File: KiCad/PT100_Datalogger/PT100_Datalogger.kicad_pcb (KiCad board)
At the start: 4 copper layers, 90 x 122 mm, 190 parts, among them J1 PWR, J10 Conn_01x03, J11 Conn_01x03, J12 Conn_01x03, J13 HLK-LD2410C, J14 691406710003B, J2 USB_C_Receptacle, J3 Screw_Terminal_01x02, J4 CT, J5 SJ1-3523N, J6 JTAG, J7 CT_SW, J8 Conn_01x03, J9 Conn_01x03, K1 J115F11CH5VDCS61.5U, Q10 BSS806NEH6327XTSA1, Q11 SSM3J36FS,LF, Q12 SSM3J36FS,LF, Q13 SSM3J36FS,LF, Q14 BSS806NEH6327XTSA1, Q15 SSM3J36FS,LF, Q16 MMBT3904, Q17 MMBT3904, Q3 BSS806NEH6327XTSA1, Q4 BSS806NEH6327XTSA1, Q5 BSS806NEH6327XTSA1, Q6 BSS806NEH6327XTSA1, Q7 BSS806NEH6327XTSA1, Q8 BSS806NEH6327XTSA1, Q9 BSS806NEH6327XTSA1, SW3 SW_Push_Shielded, SW4 SW_Push_Shielded, SW5 SW_Push_Shielded, SW6 SW_Push_Shielded, SW7 SW_Push_Shielded, U1 ESP32-S3-WROOM-1-N8R2, U10 SHT4x, U11 PCF85263AT, U12 FM24CL16B-GTR, U13 MCP9601, U2 CP2102N-Axx-xQFN28, U3 NCS2250SQ2T2G, U4 LDL212PV33R, U5 TMP1075DSG, U6 INND-TS56RAB, U7 INND-TS56RAB, U8 INND-TS56RAB, U9 INND-TS56RAB, Y1 32.768K12.5PI/3215E

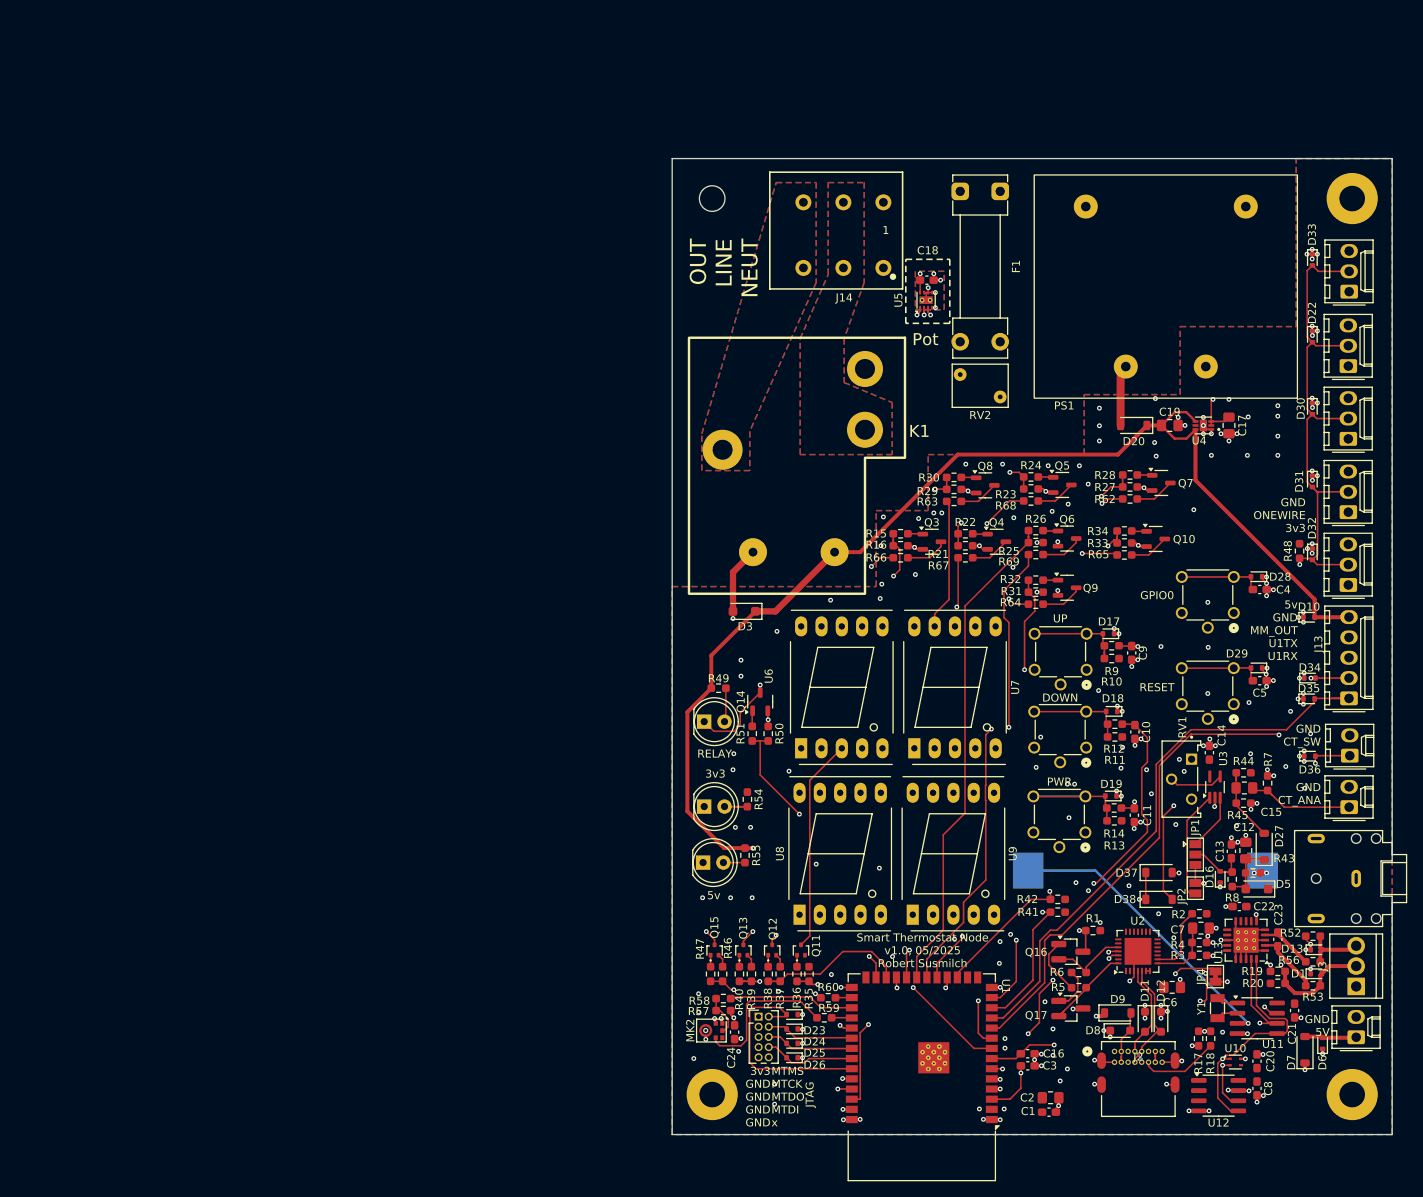
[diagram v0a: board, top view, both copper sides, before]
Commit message: Finished KiCad PCB REV A
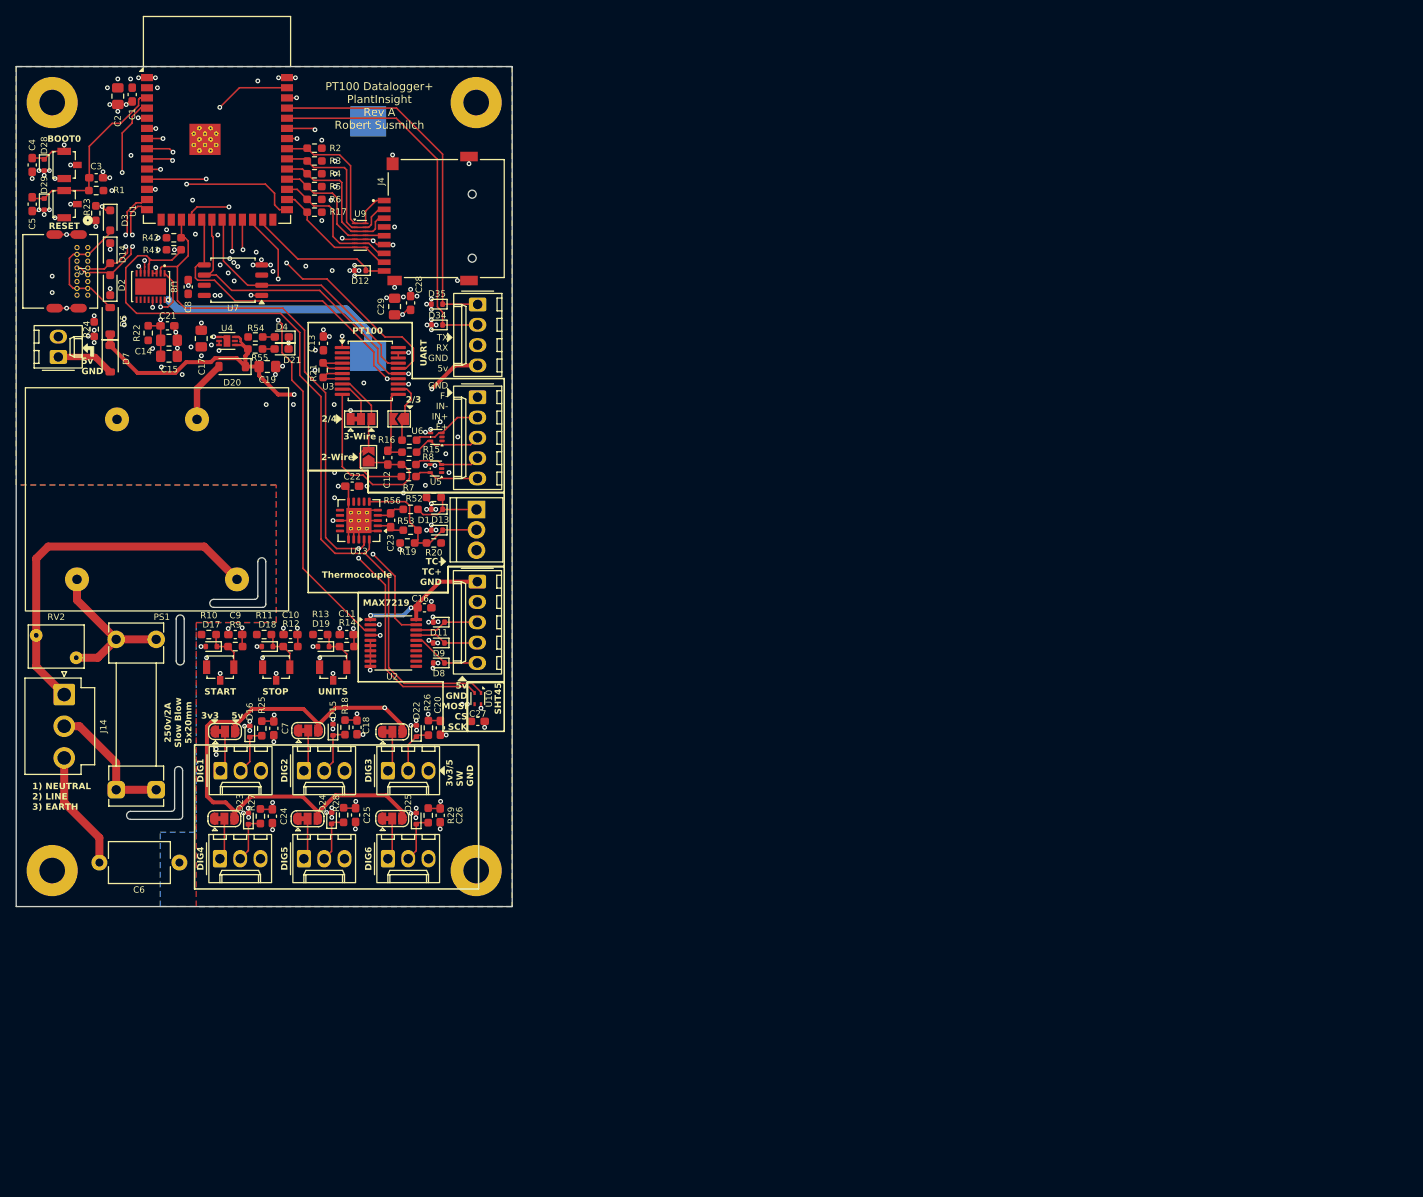
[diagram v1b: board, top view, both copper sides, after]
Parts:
- removed D10, D6: ESD5Z12T1G, Diode_SMD:D_SOD-523
- removed D26, D30, D31, D32, D33, D36: ESD5Z3V3, Diode_SMD:D_SOD-523
- removed D27, D37, D38: B5819W, Diode_SMD:D_SOD-123
- removed K1: J115F11CH5VDCS61.5U, Personal:J115FX
- removed MK2: ICS-43434, Sensor_Audio:InvenSense_ICS-43434-6_3.5x2.65mm
- removed Q10, Q14, Q3, Q4, Q5, Q6, Q7, Q8, Q9: BSS806NEH6327XTSA1, Package_TO_SOT_SMD:SOT-23-3
- removed Q11, Q12, Q13, Q15: SSM3J36FS,LF, Package_TO_SOT_SMD:SOT-416
- removed Q16, Q17: MMBT3904, Package_TO_SOT_SMD:SOT-23_Handsoldering
- removed R30, R32, R34, R36, R38, R40, R47, R51: 1K, Resistor_SMD:R_0603_1608Metric_Pad0.98x0.95mm_HandSolder
- removed R31, R33, R35, R37, R39, R46, R50, R57: 100K, Resistor_SMD:R_0603_1608Metric_Pad0.98x0.95mm_HandSolder
- removed R43: 1M, Resistor_SMD:R_0603_1608Metric_Pad0.98x0.95mm_HandSolder
- removed R44, R45: 10k, Resistor_SMD:R_0603_1608Metric_Pad0.98x0.95mm_HandSolder
- removed R48: 4K7, Resistor_SMD:R_0603_1608Metric_Pad0.98x0.95mm_HandSolder
- removed R49: 220R, Resistor_SMD:R_0603_1608Metric_Pad0.98x0.95mm_HandSolder
- removed R58, R59, R60: 51R, Resistor_SMD:R_0603_1608Metric_Pad0.98x0.95mm_HandSolder
- removed R62, R63, R64, R65, R66, R67, R68, R69: 22R, Resistor_SMD:R_0603_1608Metric_Pad0.98x0.95mm_HandSolder
- removed RV1: PV36Y102C01B00, Personal:TRIM_PV36Y102C01B00
- removed U11: PCF85263AT, Package_SO:SOIC-8_3.9x4.9mm_P1.27mm
- removed U12: FM24CL16B-GTR, Package_SO:SOIC-8_3.9x4.9mm_P1.27mm
- removed Y1: 32.768K12.5PI/3215E, Crystal:Crystal_SMD_3215-2Pin_3.2x1.5mm
- added C25: 100nF, Capacitor_SMD:C_0603_1608Metric_Pad1.08x0.95mm_HandSolder, F.Cu at (94.4, 141.1)
- added C26: 100nF, Capacitor_SMD:C_0603_1608Metric_Pad1.08x0.95mm_HandSolder, F.Cu at (105.0, 141.1)
- added C27: 100nF, Capacitor_SMD:C_0603_1608Metric_Pad1.08x0.95mm_HandSolder, F.Cu at (109.7, 129.3)
- added C28: 100nF, Capacitor_SMD:C_0603_1608Metric_Pad1.08x0.95mm_HandSolder, F.Cu at (101.3, 77.0)
- added C29: 10uF, Capacitor_SMD:C_0805_2012Metric_Pad1.18x1.45mm_HandSolder, F.Cu at (99.3, 77.5)
- added D14: TSD05CDYFR, Diode_SMD:D_SOD-323_HandSoldering, F.Cu at (63.8, 70.8)
- added D15: ESD5Z3V3, Diode_SMD:D_SOD-523, F.Cu at (91.6, 130.4)
- added JP3: SolderJumper_3_Bridged12, Jumper:SolderJumper-3_P1.3mm_Bridged12_RoundedPad1.0x1.5mm, F.Cu at (99.0, 130.7)
- added JP5: SolderJumper_3_Bridged12, Jumper:SolderJumper-3_P1.3mm_Bridged12_RoundedPad1.0x1.5mm, F.Cu at (88.4, 141.5)
- added JP6: SolderJumper_3_Bridged12, Jumper:SolderJumper-3_P1.3mm_Bridged12_RoundedPad1.0x1.5mm, F.Cu at (99.0, 141.5)
- added JP7: SolderJumper_3_Bridged12, Jumper:SolderJumper-3_P1.3mm_Bridged12_Pad1.0x1.5mm, F.Cu at (95.1, 91.6)
- added JP8: SolderJumper_2_Open, Jumper:SolderJumper-2_P1.3mm_Open_TrianglePad1.0x1.5mm, F.Cu at (99.9, 91.5)
- added JP9: SolderJumper_2_Open, Jumper:SolderJumper-2_P1.3mm_Open_TrianglePad1.0x1.5mm, F.Cu at (96.0, 96.3)
- C12, C7: value 10uF -> 100nF; footprint Capacitor_SMD:C_0805_2012Metric_Pad1.18x1.45mm_HandSolder -> Capacitor_SMD:C_0603_1608Metric_Pad1.08x0.95mm_HandSolder
- C14: value 100nF -> 22uF; footprint Capacitor_SMD:C_0603_1608Metric_Pad1.08x0.95mm_HandSolder -> Capacitor_SMD:C_0805_2012Metric_Pad1.18x1.45mm_HandSolder
- C15: value 10uF -> 22uF
- C6: value 10uF -> DE1B3RA471KN4AP01F; footprint Capacitor_SMD:C_0805_2012Metric_Pad1.18x1.45mm_HandSolder -> Capacitor_THT:C_Disc_D7.5mm_W5.0mm_P10.00mm
- D11, D8: value TSD05CDYFR -> ESD5Z12T1G; footprint Diode_SMD:D_SOD-323_HandSoldering -> Diode_SMD:D_SOD-523
- D12: value TSD05CDYFR -> ESD5Z3V3; footprint Diode_SMD:D_SOD-323_HandSoldering -> Diode_SMD:D_SOD-523
- D2: value LED -> TSD05CDYFR; footprint LED_THT:LED_D5.0mm -> Diode_SMD:D_SOD-323_HandSoldering
- D21, D4: footprint LED_THT:LED_D5.0mm -> LED_SMD:LED_0603_1608Metric_Pad1.05x0.95mm_HandSolder
- D3: value SM4007PL -> TSD05CDYFR; footprint Diode_SMD:D_SOD-123F -> Diode_SMD:D_SOD-323_HandSoldering
- D5: value SM4007PL -> B5819W; footprint Diode_SMD:D_SOD-123F -> Diode_SMD:D_SOD-123
- D9: value B5819W -> ESD5Z12T1G; footprint Diode_SMD:D_SOD-123 -> Diode_SMD:D_SOD-523
- H1: footprint MountingHole:MountingHole_3.2mm_M3 -> MountingHole:MountingHole_3.2mm_M3_Pad
- J10: value Conn_01x03 -> DIG3
- J11: value Conn_01x03 -> DIG4
- J12: value Conn_01x03 -> DIG5
- J13: value HLK-LD2410C -> DIG6; footprint Connector_Molex:Molex_KK-254_AE-6410-05A_1x05_P2.54mm_Vertical -> Connector_Molex:Molex_KK-254_AE-6410-03A_1x03_P2.54mm_Vertical
- J14: value 691406710003B -> PWR; footprint Personal:691406710003B -> Connector_JST:JST_VH_B3P-VH_1x03_P3.96mm_Vertical
- J2: value USB_C_Receptacle -> Conn_01x04; footprint Personal:CONN_CU3216SASBLR004-NH_CVI -> Connector_Molex:Molex_KK-254_AE-6410-04A_1x04_P2.54mm_Vertical
- J3: value Screw_Terminal_01x02 -> TC
- J4: value CT -> MSD-4-A; footprint Connector_Molex:Molex_KK-254_AE-6410-02A_1x02_P2.54mm_Vertical -> Personal:CUI_MSD-4-A
- J5: value SJ1-3523N -> CU3216SASBLR004-NH; footprint Connector_Audio:Jack_3.5mm_CUI_SJ1-3523N_Horizontal -> Personal:CONN_CU3216SASBLR004-NH_CVI
- J6: value JTAG -> RTD; footprint Connector_PinHeader_1.27mm:PinHeader_2x05_P1.27mm_Vertical -> Connector_Molex:Molex_KK-254_AE-6410-05A_1x05_P2.54mm_Vertical
- J7: value CT_SW -> MAX7219; footprint Connector_Molex:Molex_KK-254_AE-6410-02A_1x02_P2.54mm_Vertical -> Connector_Molex:Molex_KK-254_AE-6410-05A_1x05_P2.54mm_Vertical
- J8: value Conn_01x03 -> DIG1
- J9: value Conn_01x03 -> DIG2
- JP1: value SolderJumper_3_Open -> SolderJumper_3_Bridged12; footprint Jumper:SolderJumper-3_P1.3mm_Open_Pad1.0x1.5mm -> Jumper:SolderJumper-3_P1.3mm_Bridged12_RoundedPad1.0x1.5mm
- JP2: value SolderJumper_2_Open -> SolderJumper_3_Bridged12; footprint Jumper:SolderJumper-2_P1.3mm_Open_Pad1.0x1.5mm -> Jumper:SolderJumper-3_P1.3mm_Bridged12_RoundedPad1.0x1.5mm
- JP4: value SolderJumper_2_Bridged -> SolderJumper_3_Bridged12; footprint Jumper:SolderJumper-2_P1.3mm_Bridged_Pad1.0x1.5mm -> Jumper:SolderJumper-3_P1.3mm_Bridged12_RoundedPad1.0x1.5mm
- R15, R26, R28: value 1K -> 100R
- R16, R25, R27, R29: value 100K -> 100R
- R17: value 5k1 -> 10K
- R18: value 5k1 -> 100R
- R2: value 1K -> 10K
- R21: value 100K -> RN73H1JTTD3920A05
- R22: value 1K -> 330R
- R23: value 100K -> 5k1
- R24: value 1K -> 5k1
- R3: value 22K1 -> 10K
- R4: value 47K5 -> 10K
- R7: value 50R -> 100R
- R8: value 100 -> 100R
- SW3, SW4, SW5, SW6, SW7: footprint Personal:SW_1825955-6_TEC -> Button_Switch_SMD:SW_SPST_B3U-1100P
- U10: value SHT4x -> SHT45
- U2: value CP2102N-Axx-xQFN28 -> SN74LVC245APW; footprint Package_DFN_QFN:QFN-28-1EP_5x5mm_P0.5mm_EP3.35x3.35mm -> Package_SO:TSSOP-20_4.4x6.5mm_P0.65mm
- U3: value NCS2250SQ2T2G -> MAX31865xAP; footprint Package_TO_SOT_SMD:SOT-353_SC-70-5_Handsoldering -> Package_SO:SSOP-20_5.3x7.2mm_P0.65mm
- U5: value TMP1075DSG -> TPD2E001; footprint Package_SON:WSON-8-1EP_2x2mm_P0.5mm_EP0.9x1.6mm_ThermalVias -> Package_TO_SOT_SMD:SOT-553
- U6: value INND-TS56RAB -> TPD2E001; footprint Display_7Segment:7SegmentLED_LTS6760_LTS6780 -> Package_TO_SOT_SMD:SOT-553
- U7: value INND-TS56RAB -> CY15B104QN-50SXI; footprint Display_7Segment:7SegmentLED_LTS6760_LTS6780 -> Package_SO:SOIC-8_5.3x5.3mm_P1.27mm
- U8: value INND-TS56RAB -> PCF2131; footprint Display_7Segment:7SegmentLED_LTS6760_LTS6780 -> Personal:16-HLSON
- U9: value INND-TS56RAB -> TPD6E05U06RVZ; footprint Display_7Segment:7SegmentLED_LTS6760_LTS6780 -> Package_SON:Texas_R-PUSON-N14
- moved J1 183.2 mm to (57.3, 83.8)
- moved J5 177.1 mm to (61.0, 70.1), turned to -90 degrees
- moved D7 172.5 mm to (63.8, 84.0), turned to -90 degrees
- moved C1 171.2 mm to (66.5, 51.0), turned to -90 degrees
- moved C2 171.1 mm to (64.7, 51.2), turned to -90 degrees
- moved C8 167.0 mm to (73.5, 75.0), turned to 90 degrees
- moved H3 164.9 mm to (56.5, 148.0)
- moved C21 164.9 mm to (70.9, 79.9), turned to 0 degrees
- moved C5 164.6 mm to (54.0, 64.7), turned to -90 degrees
- moved C4 162.4 mm to (54.0, 59.8), turned to -90 degrees
- moved D29 162.3 mm to (55.5, 64.7), turned to -90 degrees
- moved C3 160.9 mm to (62.0, 61.4)
- moved D28 160.1 mm to (55.5, 59.8), turned to -90 degrees
- moved D5 160.0 mm to (63.8, 79.3), turned to 90 degrees
- moved R1 155.2 mm to (62.0, 63.0)
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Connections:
- C10 pad 1: TEMP_DOWN -> STOP
- C11 pad 1: SOFT_ON_OFF -> UNITS
- C12 pad 1: Net-(D27-K) -> Net-(JP9-A)
- C12 pad 2: GND -> Net-(JP8-B)
- C13 pad 1: Net-(D16-A2) -> +3V3
- C14 pad 1: +3V3 -> Net-(U8-IFS)
- C15 pad 1: Net-(J4-Pin_1) -> Net-(U8-IFS)
- C15 pad 2: Net-(D27-A) -> GND
- C16 pad 1: CT -> +5V
- C18 pad 1: +3V3 -> DIGITAL_2
- C20 pad 1: +3V3 -> DIGITAL_3
- C21 pad 1: +3V3 -> Net-(U8-IFS)
- C24 pad 1: +3V3 -> DIGITAL_4
- C6 pad 1: +3V3 -> Earth_Clean
- C7 pad 1: Net-(U2-VBUS) -> DIGITAL_1
- C9 pad 1: TEMP_UP -> START
- D1 pad 1: GND -> VSense
- D1 pad 2: VSense -> GND
- D11 pad 1: GND -> Net-(D11-K)
- D11 pad 2: USB_D+ -> GND
- D12 pad 1: GND -> SD_SW
- D12 pad 2: USB_D- -> GND
- D13 pad 1: GND -> Net-(D13-K)
- D13 pad 2: Net-(D13-A2) -> GND
- D16 pad 1: GND -> Net-(D16-K)
- D16 pad 2: Net-(D16-A2) -> GND
- D17 pad 1: GND -> Net-(D17-K)
- D17 pad 2: Net-(D17-A2) -> GND
- D18 pad 1: GND -> Net-(D18-K)
- D18 pad 2: Net-(D18-A2) -> GND
- D19 pad 1: GND -> Net-(D19-K)
- D19 pad 2: Net-(D19-A2) -> GND
- D2 pad 1: Net-(D2-K) -> GND
- D2 pad 2: Net-(D2-A) -> USB_D-
- D22 pad 1: GND -> Net-(D22-K)
- D22 pad 2: ONEWIRE -> GND
- D23 pad 1: GND -> Net-(D23-K)
- D23 pad 2: MTMS -> GND
- D24 pad 1: GND -> Net-(D24-K)
- D24 pad 2: MTCK -> GND
- D25 pad 1: GND -> Net-(D25-K)
- D25 pad 2: MTDO -> GND
- D28 pad 1: GND -> GPIO0
- D28 pad 2: GPIO0 -> GND
- D29 pad 1: GND -> CHIP_PU
- D29 pad 2: CHIP_PU -> GND
- D3 pad 1: +5V -> GND
- D3 pad 2: Net-(D2-K) -> VBUS
- D34 pad 1: GND -> U0RXD
- D34 pad 2: U1TX -> GND
- D35 pad 1: GND -> U0TXD
- D35 pad 2: U1RX -> GND
- D5 pad 1: +3V3 -> +5V
- D5 pad 2: Net-(D27-K) -> VBUS
- D8 pad 1: GND -> Net-(D8-K)
- D8 pad 2: VBUS -> GND
- D9 pad 1: +5V -> Net-(D9-K)
- D9 pad 2: VBUS -> GND
- H3 pad 1: GND -> unconnected-(H3-Pad1)
- J10 pad 1: +3V3 -> Net-(J10-Pin_1)
- J10 pad 2: ONEWIRE -> Net-(D22-K)
- J11 pad 1: +3V3 -> Net-(J11-Pin_1)
- J11 pad 2: ONEWIRE -> Net-(D23-K)
- J12 pad 1: +3V3 -> Net-(J12-Pin_1)
- J12 pad 2: ONEWIRE -> Net-(D24-K)
- J13 pad 1: U1RX -> Net-(J13-Pin_1)
- J13 pad 2: U1TX -> Net-(D25-K)
- J13 pad 3: MM_OUT -> GND
- J14 pad 3: AC_OUT -> Earth_Clean
- J3 pad 1: GND -> Net-(D13-K)
- J3 pad 3: Net-(D13-A2) -> GND
- J4 pad 1: Net-(J4-Pin_1) -> SD_D2
- J4 pad 2: GND -> SD_D3
- J6 pad 1: +3V3 -> GND
- J6 pad 2: MTMS -> RTD_FN
- J6 pad 3: GND -> RTD_INN
- J6 pad 4: MTCK -> RTD_INP
- J6 pad 5: GND -> RTD_FP
- J7 pad 1: CT -> +5V
- J8 pad 1: +3V3 -> Net-(J8-Pin_1)
- J8 pad 2: ONEWIRE -> Net-(D16-K)
- J9 pad 1: +3V3 -> Net-(J9-Pin_1)
- J9 pad 2: ONEWIRE -> Net-(D15-K)
- JP1 pad 1: Net-(JP1-A) -> +3V3
- JP1 pad 2: Net-(D16-A2) -> Net-(J8-Pin_1)
- JP1 pad 3: CT -> +5V
- JP2 pad 1: Net-(JP2-A) -> +3V3
- JP2 pad 2: CT -> Net-(J9-Pin_1)
- JP4 pad 1: Net-(JP4-A) -> +3V3
- JP4 pad 2: CHIP_PU -> Net-(J11-Pin_1)
- R10 pad 1: Net-(D17-A2) -> Net-(D17-K)
- R11 pad 1: Net-(D18-A2) -> Net-(D18-K)
- R12 pad 1: Net-(D18-A2) -> Net-(D18-K)
- R12 pad 2: TEMP_DOWN -> STOP
- R13 pad 1: Net-(D19-A2) -> Net-(D19-K)
- R14 pad 1: Net-(D19-A2) -> Net-(D19-K)
- R14 pad 2: SOFT_ON_OFF -> UNITS
- R15 pad 1: SEG_A -> Net-(JP8-B)
- R15 pad 2: Net-(Q3-G) -> RTD_INN
- R16 pad 1: GND -> Net-(JP8-A)
- R16 pad 2: SEG_A -> RTD_FN
- R17 pad 1: Net-(J2-CC1) -> +3V3
- R17 pad 2: GND -> SD_D1
- R18 pad 1: Net-(J2-CC2) -> Net-(D15-K)
- R18 pad 2: GND -> DIGITAL_2
- R2 pad 2: Net-(U2-~{RST}) -> SD_D2
- R21 pad 1: GND -> Net-(U3-BIAS)
- R21 pad 2: SEG_B -> Net-(U3-ISENSOR)
- R22 pad 1: SEG_B -> +3V3
- R22 pad 2: Net-(Q4-G) -> Net-(U8-IFS)
- R23 pad 1: GND -> Net-(J5-CC1)
- R23 pad 2: SEG_C -> GND
- R24 pad 1: SEG_C -> Net-(J5-CC2)
- R24 pad 2: Net-(Q5-G) -> GND
- R25 pad 1: GND -> Net-(D16-K)
- R25 pad 2: SEG_D -> DIGITAL_1
- R26 pad 1: SEG_D -> Net-(D22-K)
- R26 pad 2: Net-(Q6-G) -> DIGITAL_3
- R27 pad 1: GND -> Net-(D23-K)
- R27 pad 2: SEG_E -> DIGITAL_4
- R28 pad 1: SEG_E -> Net-(D24-K)
- R28 pad 2: Net-(Q7-G) -> DIGITAL_5
- R29 pad 1: GND -> Net-(D25-K)
- R29 pad 2: SEG_F -> DIGITAL_6
- R3 pad 1: VBUS -> +3V3
- R3 pad 2: Net-(U2-VBUS) -> SD_D3
- R4 pad 1: Net-(U2-VBUS) -> +3V3
- R4 pad 2: GND -> SD_CMD
- R5 pad 1: DTR -> +3V3
- R5 pad 2: Net-(Q16-B) -> SD_CLK
- R52 pad 1: Net-(D13-A2) -> Net-(D13-K)
- R56 pad 1: Net-(D13-A2) -> Net-(D13-K)
- R6 pad 1: RTS -> +3V3
- R6 pad 2: Net-(Q17-B) -> SD_D0
- R7 pad 1: Net-(J4-Pin_1) -> Net-(JP7-B)
- R7 pad 2: GND -> RTD_FP
- R8 pad 1: Net-(D27-K) -> Net-(JP9-A)
- R8 pad 2: Net-(D16-A2) -> RTD_INP
- R9 pad 1: Net-(D17-A2) -> Net-(D17-K)
- R9 pad 2: TEMP_UP -> START
- SW3 pad 2: Net-(D17-A2) -> Net-(D17-K)
- SW4 pad 2: Net-(D18-A2) -> Net-(D18-K)
- SW5 pad 2: Net-(D19-A2) -> Net-(D19-K)
- U1 pad 10: U1TX -> DIGITAL_4
- U1 pad 11: U1RX -> LEVEL_OE
- U1 pad 13: SEG_DP -> USB_D-
- U1 pad 14: ALERT -> USB_D+
- U1 pad 18: SEG_A -> MAX_CS
- U1 pad 19: SEG_B -> MOSI
- U1 pad 20: SEG_C -> SCK
- U1 pad 21: SEG_D -> MISO
- U1 pad 22: SEG_E -> DIGITAL_2
- U1 pad 23: DIG_1 -> DIGITAL_5
- U1 pad 24: DIG_2 -> D_CS
- U1 pad 25: DIG_3 -> SD_SW
- U1 pad 28: Net-(U1-IO35) -> SD_D1
- U1 pad 29: I2S_D -> SD_D0
- U1 pad 30: Net-(U1-IO37) -> SD_CLK
- U1 pad 31: RELAY_PWR -> SD_CMD
- U1 pad 32: MTCK -> SD_D3
- U1 pad 33: MTDO -> SD_D2
- U1 pad 34: MTDI -> ~{MAX_RDY}
- U1 pad 35: MTMS -> DIGITAL_6
- U1 pad 38: DIG_4 -> RTC_INT
- U1 pad 39: ONEWIRE -> 1HZ
- U1 pad 4: SOFT_ON_OFF -> DIGITAL_1
- U1 pad 5: TEMP_DOWN -> START
- U1 pad 6: TEMP_UP -> STOP
- U1 pad 7: CT -> UNITS
- U1 pad 8: SEG_F -> FRAM_CS
- U1 pad 9: SEG_G -> DIGITAL_3
- U2 pad 1: unconnected-(U2-~{DCD}-Pad1) -> +5V
- U2 pad 10: unconnected-(U2-NC-Pad10) -> GND
- U2 pad 16: unconnected-(U2-~{WAKEUP}/GPIO.3-Pad16) -> Net-(D8-K)
- U2 pad 17: unconnected-(U2-RS485/GPIO.2-Pad17) -> Net-(D9-K)
- U2 pad 18: unconnected-(U2-~{RXT}/GPIO.1-Pad18) -> Net-(D11-K)
- U2 pad 19: unconnected-(U2-~{TXT}/GPIO.0-Pad19) -> LEVEL_OE
- U2 pad 2: unconnected-(U2-~{RI}/CLK-Pad2) -> MOSI
- U2 pad 20: unconnected-(U2-GPIO.6-Pad20) -> +5V
- U2 pad 3: GND -> D_CS
- U2 pad 4: USB_D+ -> SCK
- U2 pad 5: USB_D- -> GND
- U2 pad 6: +3V3 -> GND
- U2 pad 7: +3V3 -> GND
- U2 pad 8: Net-(U2-VBUS) -> GND
- U2 pad 9: Net-(U2-~{RST}) -> GND
- U3 pad 1: Net-(JP2-A) -> ~{MAX_RDY}
- U3 pad 2: GND -> +3V3
- U3 pad 3: Net-(JP1-A) -> +3V3
- U3 pad 4: Net-(U3--) -> Net-(U3-BIAS)
- U3 pad 5: +3V3 -> Net-(U3-BIAS)
- U5 pad 1: SDA -> +3V3
- U5 pad 2: SCL -> unconnected-(U5-NC-Pad2)
- U5 pad 3: RELAY_ALERT -> RTD_INP
- U5 pad 5: GND -> RTD_FP
- U6 pad 1: SEG_E_LED -> +3V3
- U6 pad 2: SEG_D_LED -> unconnected-(U6-NC-Pad2)
- U6 pad 3: DIG_1_LED -> RTD_FN
- U6 pad 4: SEG_C_LED -> GND
- U6 pad 5: SEG_DP_LED -> RTD_INN
- U7 pad 1: SEG_E_LED -> FRAM_CS
- U7 pad 2: SEG_D_LED -> MISO
- U7 pad 3: DIG_2_LED -> +3V3
- U7 pad 4: SEG_C_LED -> GND
- U7 pad 5: SEG_DP_LED -> MOSI
- U7 pad 6: SEG_B_LED -> SCK
- U7 pad 7: SEG_A_LED -> unconnected-(U7-~{HOLD}-Pad7)
- U7 pad 8: DIG_2_LED -> +3V3
- U8 pad 1: SEG_E_LED -> Net-(U8-IFS)
- U8 pad 10: SEG_G_LED -> unconnected-(U8-~{TS3}-Pad10)
- U8 pad 2: SEG_D_LED -> SCL
- U8 pad 3: DIG_3_LED -> GND
- U8 pad 4: SEG_C_LED -> GND
- U8 pad 5: SEG_DP_LED -> SDA
- U8 pad 6: SEG_B_LED -> 1HZ
- U8 pad 7: SEG_A_LED -> GND
- U8 pad 8: DIG_3_LED -> unconnected-(U8-~{TS1}-Pad8)
- U8 pad 9: SEG_F_LED -> unconnected-(U8-~{TS2}-Pad9)
- U9 pad 1: SEG_E_LED -> SD_D2
- U9 pad 10: SEG_G_LED -> GND
- U9 pad 2: SEG_D_LED -> SD_D3
- U9 pad 3: DIG_4_LED -> SD_CMD
- U9 pad 4: SEG_C_LED -> SD_CLK
- U9 pad 5: SEG_DP_LED -> GND
- U9 pad 6: SEG_B_LED -> SD_D0
- U9 pad 7: SEG_A_LED -> SD_D1
- U9 pad 8: DIG_4_LED -> SD_D1
- U9 pad 9: SEG_F_LED -> SD_D0
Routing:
- net ONEWIRE: track 163.7 -> 0.00 mm, vias 2 -> 0
- net SEG_E_LED: track 116.2 -> 0.00 mm, vias 2 -> 0
- net DIGITAL_4: track 0.00 -> 102.3 mm, vias 0 -> 2
- net DIGITAL_6: track 0.00 -> 99.2 mm, vias 0 -> 2
- net DIGITAL_1: track 0.00 -> 98.3 mm, vias 0 -> 2
- net SEG_C_LED: track 95.7 -> 0.00 mm, vias 1 -> 0
- net SEG_D_LED: track 94.7 -> 0.00 mm, vias 1 -> 0
- net SEG_DP_LED: track 94.6 -> 0.00 mm, vias 1 -> 0
- net DIGITAL_3: track 0.00 -> 93.8 mm, vias 0 -> 2
- net RELAY_ALERT: track 87.0 -> 0.00 mm, vias 2 -> 0
- net START: track 0.00 -> 87.0 mm, vias 0 -> 2
- net UNITS: track 0.00 -> 86.7 mm, vias 0 -> 2
- net STOP: track 0.00 -> 85.0 mm, vias 0 -> 2
- net DIGITAL_5: track 0.00 -> 81.8 mm, vias 0 -> 2
- net SEG_E: track 80.9 -> 0.00 mm, vias 3 -> 0
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- removed copper zone on B.Cu, net AC_OUT
- removed copper zone on F.Cu, net AC_OUT
- removed copper zone on In1.Cu, net AC_OUT
- removed copper zone on In2.Cu, net AC_OUT
- removed copper zone on F.Cu, net GND
- removed copper zone on In2.Cu, net GND
- removed copper zone on B.Cu, net L1
- removed copper zone on F.Cu, net L1
- removed copper zone on In1.Cu, net L1
- removed copper zone on In2.Cu, net L1
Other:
- board size 90 x 122 mm -> 62 x 105 mm
- board text added: "1) NEUTRAL 2) LINE 3) EARTH"
- board text added: "2-Wire"
- board text added: "2/3"
- board text added: "2/4"
- board text added: "250v/2A Slow Blow 5x20mm"
- board text added: "3-Wire"
- board text added: "3v3/5 SW GND"
- board text added: "5v GND"
- board text added: "5v GND MOSI CS SCK"
- board text added: "BOOT0"
- board text added: "DIG1"
- board text added: "DIG2"
- board text added: "DIG3"
- board text added: "DIG4"
- board text added: "DIG5"
- board text added: "DIG6"
- board text added: "GND F- IN- IN+ F+"
- board text added: "MAX7219"
- board text added: "PT100"
- board text added: "PT100 Datalogger+ PlantInsight Rev A Robert Susmilch"
- board text added: "SHT45"
- board text added: "START"
- board text added: "STOP"
- board text added: "TC- TC+ GND"
- board text added: "TX RX GND 5v"
- board text added: "Thermocouple"
- board text added: "UART"
- board text added: "UNITS"
- board text removed: "3v3 GND GND GND GND"
- board text removed: "5v GND MM_OUT U1TX U1RX"
- board text removed: "DOWN"
- board text removed: "GND 5V"
- board text removed: "GND CT_ANA"
- board text removed: "GND CT_SW"
- board text removed: "GND ONEWIRE 3v3"
- board text removed: "GPIO0"
- board text removed: "JLCJLCJLCJLC"
- board text removed: "JTAG"
- board text removed: "MTMS MTCK MTDO MTDI x"
- board text removed: "OUT LINE NEUT"
- board text removed: "PWR"
- board text removed: "Pot"
- board text removed: "RELAY"
- board text removed: "Smart Thermostat Node v1.0, 05/2025 Robert Susmilch"
- board text removed: "UP"
